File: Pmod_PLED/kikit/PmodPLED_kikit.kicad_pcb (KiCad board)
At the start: 2 copper layers, 86.5 x 99.3 mm, 148 parts, among them IC1 TBD62064APG, IC2 LM2940T-5.0, J1 Barrel_Jack_Switch, J2 Conn_01x06_Pin, J3 Conn_01x03_Pin

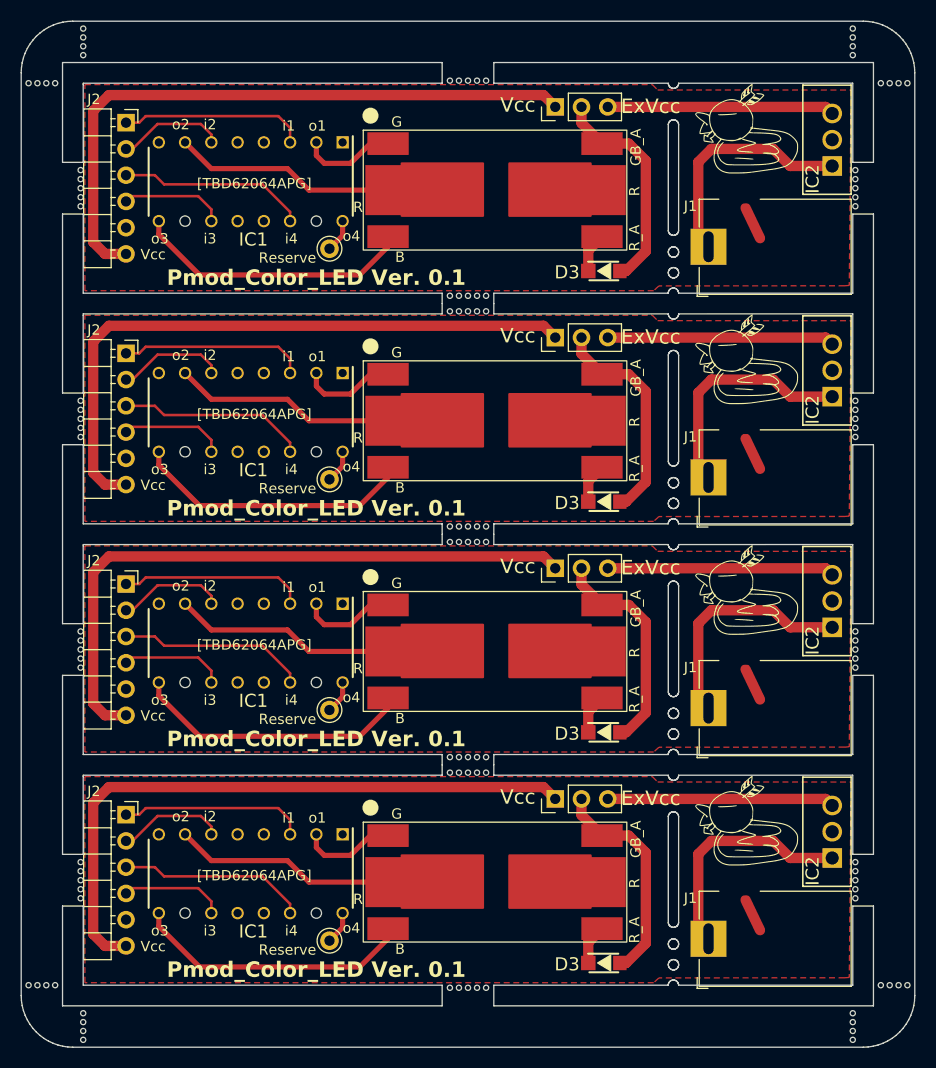
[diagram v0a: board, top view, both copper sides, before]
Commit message: 601d
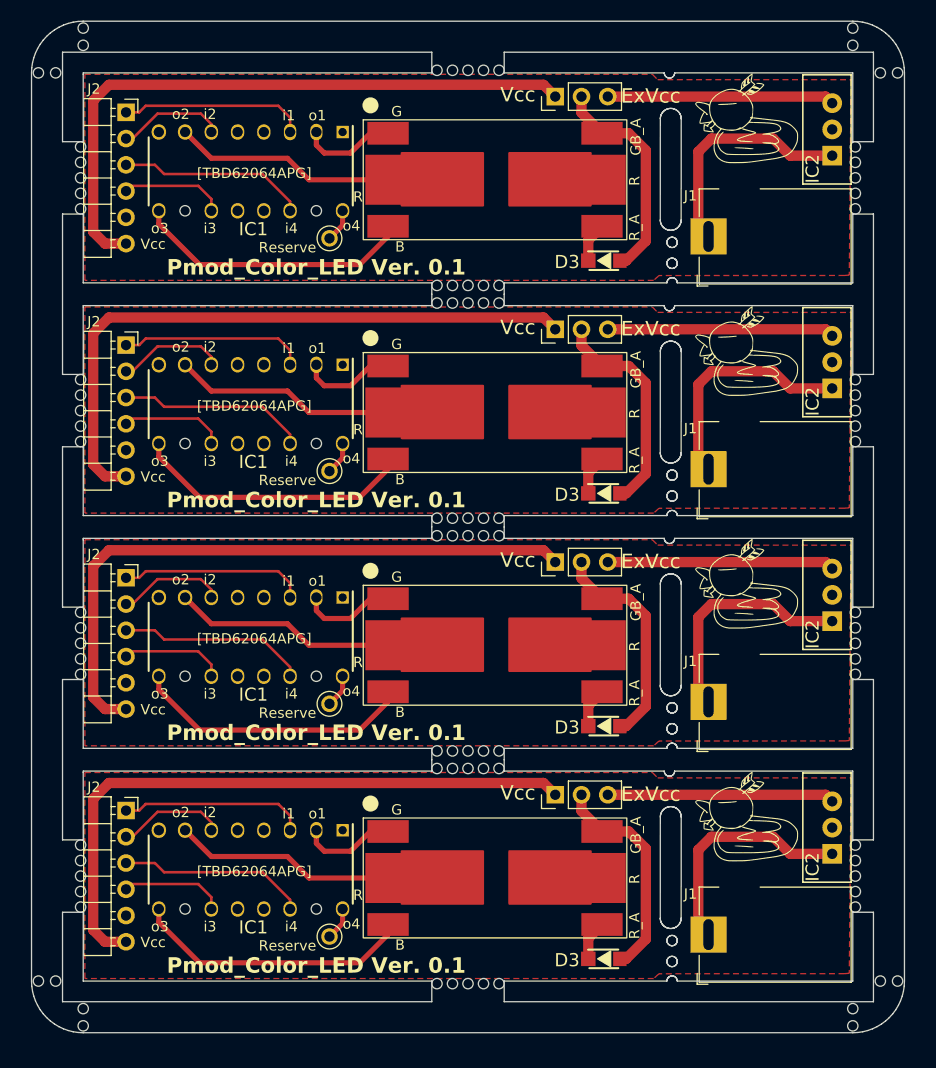
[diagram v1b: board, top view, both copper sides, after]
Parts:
- removed the D1 at (151.2, 36.3)
- removed the D1 at (151.2, 103.3)
- removed the D1 at (151.2, 81.0)
- removed the D1 at (151.2, 58.7)
- removed the D3 at (161.6, 66.5)
- removed the D3 at (161.6, 111.1)
- removed the D3 at (161.6, 88.8)
- removed the D3 at (161.6, 44.2)
- removed the G*** at (175.4, 97.4)
- removed the G*** at (175.4, 75.1)
- removed the G*** at (175.4, 30.5)
- removed the G*** at (175.4, 52.8)
- removed the IC1 at (127.5, 80.2)
- removed the IC1 at (127.5, 35.5)
- removed the IC1 at (127.5, 102.5)
- removed the IC1 at (127.5, 57.9)
- removed the IC2 at (182.7, 95.9)
- removed the IC2 at (182.7, 51.2)
- removed the IC2 at (182.7, 28.9)
- removed the IC2 at (182.7, 73.6)
- removed the J1 at (171.8, 64.1)
- removed the J1 at (171.8, 86.5)
- removed the J1 at (171.8, 108.8)
- removed the J1 at (171.8, 41.8)
- removed the J2 at (111.4, 95.5)
- removed the J2 at (111.4, 73.2)
- removed the J2 at (111.4, 50.9)
- removed the J2 at (111.4, 28.5)
- removed the J3 at (156.9, 28.3)
- removed the J3 at (156.9, 72.9)
- removed the J3 at (156.9, 95.2)
- removed the J3 at (156.9, 50.6)
- removed the REF** at (111.0, 35.3)
- removed the REF** at (186.0, 103.1)
- removed the REF** at (147.6, 70.4)
- removed the REF** at (111.3, 118.6)
- removed the REF** at (150.2, 46.6)
- removed the REF** at (185.7, 118.6)
- removed the REF** at (111.0, 60.2)
- removed the REF** at (111.3, 116.8)
- removed the REF** at (189.3, 113.3)
- removed the REF** at (106.8, 26.0)
- removed the REF** at (149.4, 48.1)
- removed the REF** at (108.6, 113.3)
- removed the REF** at (111.0, 37.0)
- removed the REF** at (186.0, 60.2)
- removed the REF** at (150.2, 92.7)
- removed the REF** at (186.0, 56.7)
- removed the REF** at (150.2, 113.5)
- removed the REF** at (185.7, 23.3)
- removed the REF** at (111.0, 82.5)
- removed the REF** at (108.6, 26.0)
- removed the REF** at (111.0, 102.2)
- removed the REF** at (111.0, 57.6)
- removed the REF** at (147.6, 25.8)
- removed the REF** at (146.8, 70.4)
- removed the REF** at (186.0, 37.9)
- removed the REF** at (189.3, 26.0)
- removed the REF** at (146.8, 25.8)
- removed the REF** at (111.3, 22.4)
- removed the REF** at (107.7, 26.0)
- removed the REF** at (111.3, 23.3)
- removed the REF** at (186.0, 79.0)
- removed the REF** at (111.0, 81.7)
- removed the REF** at (186.0, 59.4)
- removed the REF** at (106.8, 113.3)
- removed the REF** at (185.7, 116.0)
- removed the REF** at (149.4, 70.4)
- removed the REF** at (185.7, 117.7)
- removed the REF** at (148.5, 46.6)
- removed the REF** at (147.6, 48.1)
- removed the REF** at (186.0, 58.5)
- removed the REF** at (111.3, 20.7)
- removed the REF** at (111.0, 79.0)
- removed the REF** at (186.0, 101.4)
- removed the REF** at (111.0, 59.4)
- removed the REF** at (148.5, 113.5)
- removed the REF** at (186.0, 80.8)
- removed the REF** at (186.0, 102.2)
- removed the REF** at (185.7, 20.7)
- removed the REF** at (186.0, 36.2)
- removed the REF** at (146.8, 68.9)
- removed the REF** at (186.0, 104.0)
- removed the REF** at (149.4, 46.6)
- removed the REF** at (147.6, 68.9)
- removed the REF** at (148.5, 91.2)
- removed the REF** at (149.4, 91.2)
- removed the REF** at (185.7, 22.4)
- removed the REF** at (186.0, 37.0)
- removed the REF** at (186.0, 81.7)
- removed the REF** at (106.0, 26.0)
- removed the REF** at (147.6, 91.2)
- removed the REF** at (146.8, 91.2)
- removed the REF** at (186.0, 34.4)
- removed the REF** at (111.3, 117.7)
- removed the REF** at (111.0, 37.9)
- removed the REF** at (191.0, 113.3)
- removed the REF** at (188.4, 26.0)
- removed the REF** at (190.2, 26.0)
- removed the REF** at (146.8, 92.7)
- removed the REF** at (148.5, 25.8)
- removed the REF** at (147.6, 92.7)
- removed the REF** at (185.7, 21.6)
- removed the REF** at (186.0, 82.5)
- removed the REF** at (150.2, 70.4)
- removed the REF** at (111.3, 116.0)
- removed the REF** at (146.8, 48.1)
- removed the REF** at (106.0, 113.3)
- removed the REF** at (107.7, 113.3)
- removed the REF** at (111.3, 21.6)
- removed the REF** at (111.0, 34.4)
- removed the REF** at (190.2, 113.3)
- removed the REF** at (147.6, 113.5)
- removed the REF** at (185.7, 116.8)
- removed the REF** at (148.5, 48.1)
- removed the REF** at (191.0, 26.0)
- removed the REF** at (111.0, 36.2)
- removed the REF** at (186.0, 79.9)
- removed the REF** at (186.0, 57.6)
- removed the REF** at (111.0, 80.8)
- removed the REF** at (186.0, 35.3)
- removed the REF** at (147.6, 46.6)
- removed the REF** at (146.8, 46.6)
- removed the REF** at (146.8, 113.5)
- removed the REF** at (111.0, 56.7)
- removed the REF** at (111.0, 58.5)
- removed the REF** at (111.0, 104.9)
- removed the REF** at (150.2, 68.9)
- removed the REF** at (150.2, 48.1)
- removed the REF** at (148.5, 70.4)
- removed the REF** at (149.4, 92.7)
- removed the REF** at (111.0, 103.1)
- removed the REF** at (111.0, 101.4)
- removed the REF** at (149.4, 68.9)
- removed the REF** at (111.0, 104.0)
- removed the REF** at (188.4, 113.3)
- removed the REF** at (186.0, 104.9)
- removed the REF** at (111.0, 79.9)
- removed the REF** at (149.4, 25.8)
- removed the REF** at (150.2, 25.8)
- removed the REF** at (148.5, 68.9)
- removed the REF** at (148.5, 92.7)
- removed the REF** at (149.4, 113.5)
- removed the REF** at (150.2, 91.2)
- removed the Reserve at (135.1, 109.0)
- removed the Reserve at (135.1, 64.3)
- removed the Reserve at (135.1, 86.6)
- removed the Reserve at (135.1, 42.0)
- added D1: EP204K-150G1R1B1-CA, MyLibrary:EP204-150G1R1B1-CA, F.Cu at (151.2, 102.9)
- added D1: EP204K-150G1R1B1-CA, MyLibrary:EP204-150G1R1B1-CA, F.Cu at (151.2, 35.3)
- added D1: EP204K-150G1R1B1-CA, MyLibrary:EP204-150G1R1B1-CA, F.Cu at (151.2, 57.9)
- added D1: EP204K-150G1R1B1-CA, MyLibrary:EP204-150G1R1B1-CA, F.Cu at (151.2, 80.4)
- added D3: SS2040FL, SamacSys_Parts:SODFL3618X108N, F.Cu at (161.6, 110.7)
- added D3: SS2040FL, SamacSys_Parts:SODFL3618X108N, F.Cu at (161.6, 43.2)
- added D3: SS2040FL, SamacSys_Parts:SODFL3618X108N, F.Cu at (161.6, 88.2)
- added D3: SS2040FL, SamacSys_Parts:SODFL3618X108N, F.Cu at (161.6, 65.7)
- added G***: LOGO, MyLibrary:logo_kamo_ss, F.Cu at (175.4, 74.5)
- added G***: LOGO, MyLibrary:logo_kamo_ss, F.Cu at (175.4, 97.0)
- added G***: LOGO, MyLibrary:logo_kamo_ss, F.Cu at (175.4, 52.0)
- added G***: LOGO, MyLibrary:logo_kamo_ss, F.Cu at (175.4, 29.5)
- added IC1: TBD62064APG, SamacSys_Parts:DIP762W60P254L1975H445Q16N, F.Cu at (127.5, 34.5)
- added IC1: TBD62064APG, SamacSys_Parts:DIP762W60P254L1975H445Q16N, F.Cu at (127.5, 79.6)
- added IC1: TBD62064APG, SamacSys_Parts:DIP762W60P254L1975H445Q16N, F.Cu at (127.5, 57.1)
- added IC1: TBD62064APG, SamacSys_Parts:DIP762W60P254L1975H445Q16N, F.Cu at (127.5, 102.1)
- added IC2: LM2940T-5.0, SamacSys_Parts:TO254P470X1016X2222-3P, F.Cu at (182.7, 95.5)
- added IC2: LM2940T-5.0, SamacSys_Parts:TO254P470X1016X2222-3P, F.Cu at (182.7, 50.4)
- added IC2: LM2940T-5.0, SamacSys_Parts:TO254P470X1016X2222-3P, F.Cu at (182.7, 27.9)
- added IC2: LM2940T-5.0, SamacSys_Parts:TO254P470X1016X2222-3P, F.Cu at (182.7, 73.0)
- added J1: Barrel_Jack_Switch, Connector_BarrelJack:BarrelJack_Horizontal, F.Cu at (171.8, 63.3)
- added J1: Barrel_Jack_Switch, Connector_BarrelJack:BarrelJack_Horizontal, F.Cu at (171.8, 108.4)
- added J1: Barrel_Jack_Switch, Connector_BarrelJack:BarrelJack_Horizontal, F.Cu at (171.8, 85.9)
- added J1: Barrel_Jack_Switch, Connector_BarrelJack:BarrelJack_Horizontal, F.Cu at (171.8, 40.8)
- added J2: Conn_01x06_Pin, Library:Pmod6, F.Cu at (111.4, 72.6)
- added J2: Conn_01x06_Pin, Library:Pmod6, F.Cu at (111.4, 50.1)
- added J2: Conn_01x06_Pin, Library:Pmod6, F.Cu at (111.4, 95.1)
- added J2: Conn_01x06_Pin, Library:Pmod6, F.Cu at (111.4, 27.5)
- added J3: Conn_01x03_Pin, Connector_PinHeader_2.54mm:PinHeader_1x03_P2.54mm_Vertical, F.Cu at (156.9, 94.8)
- added J3: Conn_01x03_Pin, Connector_PinHeader_2.54mm:PinHeader_1x03_P2.54mm_Vertical, F.Cu at (156.9, 49.8)
- added J3: Conn_01x03_Pin, Connector_PinHeader_2.54mm:PinHeader_1x03_P2.54mm_Vertical, F.Cu at (156.9, 27.3)
- added J3: Conn_01x03_Pin, Connector_PinHeader_2.54mm:PinHeader_1x03_P2.54mm_Vertical, F.Cu at (156.9, 72.3)
- added REF**: NPTH, NPTH, F.Cu at (186.0, 59.2)
- added REF**: NPTH, NPTH, F.Cu at (186.0, 60.7)
- added REF**: NPTH, NPTH, F.Cu at (186.0, 33.7)
- added REF**: NPTH, NPTH, F.Cu at (111.0, 35.2)
- added REF**: NPTH, NPTH, F.Cu at (150.0, 24.8)
- added REF**: NPTH, NPTH, F.Cu at (185.7, 115.5)
- added REF**: NPTH, NPTH, F.Cu at (150.0, 68.1)
- added REF**: NPTH, NPTH, F.Cu at (190.1, 25.0)
- added REF**: NPTH, NPTH, F.Cu at (111.3, 20.7)
- added REF**: NPTH, NPTH, F.Cu at (111.0, 99.7)
- added REF**: NPTH, NPTH, F.Cu at (111.0, 56.2)
- added REF**: NPTH, NPTH, F.Cu at (145.5, 90.6)
- added REF**: NPTH, NPTH, F.Cu at (111.0, 57.7)
- added REF**: NPTH, NPTH, F.Cu at (106.9, 25.0)
- added REF**: NPTH, NPTH, F.Cu at (111.0, 105.7)
- added REF**: NPTH, NPTH, F.Cu at (151.5, 24.8)
- added REF**: NPTH, NPTH, F.Cu at (111.0, 78.7)
- added REF**: NPTH, NPTH, F.Cu at (111.3, 117.2)
- added REF**: NPTH, NPTH, F.Cu at (150.0, 45.6)
- added REF**: NPTH, NPTH, F.Cu at (147.0, 69.8)
- added REF**: NPTH, NPTH, F.Cu at (185.7, 22.3)
- added REF**: NPTH, NPTH, F.Cu at (151.5, 47.3)
- added REF**: NPTH, NPTH, F.Cu at (186.0, 36.7)
- added REF**: NPTH, NPTH, F.Cu at (186.0, 56.2)
- added REF**: NPTH, NPTH, F.Cu at (148.5, 92.3)
- added REF**: NPTH, NPTH, F.Cu at (148.5, 45.6)
- added REF**: NPTH, NPTH, F.Cu at (147.0, 92.3)
- added REF**: NPTH, NPTH, F.Cu at (147.0, 24.8)
- added REF**: NPTH, NPTH, F.Cu at (145.5, 45.6)
- added REF**: NPTH, NPTH, F.Cu at (147.0, 45.6)
- added REF**: NPTH, NPTH, F.Cu at (150.0, 92.3)
- added REF**: NPTH, NPTH, F.Cu at (188.4, 112.9)
- added REF**: NPTH, NPTH, F.Cu at (106.9, 112.9)
- added REF**: NPTH, NPTH, F.Cu at (145.5, 92.3)
- added REF**: NPTH, NPTH, F.Cu at (186.0, 99.7)
- added REF**: NPTH, NPTH, F.Cu at (145.5, 113.1)
- added REF**: NPTH, NPTH, F.Cu at (111.3, 22.3)
- added REF**: NPTH, NPTH, F.Cu at (111.0, 81.7)
- added REF**: NPTH, NPTH, F.Cu at (186.0, 101.2)
- added REF**: NPTH, NPTH, F.Cu at (111.3, 115.5)
- added REF**: NPTH, NPTH, F.Cu at (151.5, 69.8)
- added REF**: NPTH, NPTH, F.Cu at (188.4, 25.0)
- added REF**: NPTH, NPTH, F.Cu at (111.0, 59.2)
- added REF**: NPTH, NPTH, F.Cu at (186.0, 105.7)
- added REF**: NPTH, NPTH, F.Cu at (148.5, 69.8)
- added REF**: NPTH, NPTH, F.Cu at (147.0, 90.6)
- added REF**: NPTH, NPTH, F.Cu at (147.0, 47.3)
- added REF**: NPTH, NPTH, F.Cu at (186.0, 78.7)
- added REF**: NPTH, NPTH, F.Cu at (150.0, 47.3)
- added REF**: NPTH, NPTH, F.Cu at (111.0, 54.7)
- added REF**: NPTH, NPTH, F.Cu at (186.0, 35.2)
- added REF**: NPTH, NPTH, F.Cu at (145.5, 69.8)
- added REF**: NPTH, NPTH, F.Cu at (111.0, 83.2)
- added REF**: NPTH, NPTH, F.Cu at (111.0, 104.2)
- added REF**: NPTH, NPTH, F.Cu at (151.5, 90.6)
- added REF**: NPTH, NPTH, F.Cu at (111.0, 80.2)
- added REF**: NPTH, NPTH, F.Cu at (111.0, 102.7)
- added REF**: NPTH, NPTH, F.Cu at (111.0, 60.7)
- added REF**: NPTH, NPTH, F.Cu at (186.0, 38.2)
- added REF**: NPTH, NPTH, F.Cu at (145.5, 24.8)
- added REF**: NPTH, NPTH, F.Cu at (111.0, 32.2)
- added REF**: NPTH, NPTH, F.Cu at (148.5, 90.6)
- added REF**: NPTH, NPTH, F.Cu at (186.0, 102.7)
- added REF**: NPTH, NPTH, F.Cu at (108.6, 112.9)
- added REF**: NPTH, NPTH, F.Cu at (186.0, 80.2)
- added REF**: NPTH, NPTH, F.Cu at (151.5, 92.3)
- added REF**: NPTH, NPTH, F.Cu at (150.0, 90.6)
- added REF**: NPTH, NPTH, F.Cu at (145.5, 68.1)
- added REF**: NPTH, NPTH, F.Cu at (186.0, 81.7)
- added REF**: NPTH, NPTH, F.Cu at (186.0, 32.2)
- added REF**: NPTH, NPTH, F.Cu at (148.5, 113.1)
- added REF**: NPTH, NPTH, F.Cu at (190.1, 112.9)
- added REF**: NPTH, NPTH, F.Cu at (145.5, 47.3)
- added REF**: NPTH, NPTH, F.Cu at (151.5, 113.1)
- added REF**: NPTH, NPTH, F.Cu at (185.7, 117.2)
- added REF**: NPTH, NPTH, F.Cu at (111.0, 38.2)
- added REF**: NPTH, NPTH, F.Cu at (111.0, 36.7)
- added REF**: NPTH, NPTH, F.Cu at (147.0, 68.1)
- added REF**: NPTH, NPTH, F.Cu at (108.6, 25.0)
- added REF**: NPTH, NPTH, F.Cu at (151.5, 68.1)
- added REF**: NPTH, NPTH, F.Cu at (186.0, 83.2)
- added REF**: NPTH, NPTH, F.Cu at (186.0, 104.2)
- added REF**: NPTH, NPTH, F.Cu at (151.5, 45.6)
- added REF**: NPTH, NPTH, F.Cu at (148.5, 68.1)
- added REF**: NPTH, NPTH, F.Cu at (111.0, 33.7)
- added REF**: NPTH, NPTH, F.Cu at (148.5, 47.3)
- added REF**: NPTH, NPTH, F.Cu at (150.0, 69.8)
- added REF**: NPTH, NPTH, F.Cu at (150.0, 113.1)
- added REF**: NPTH, NPTH, F.Cu at (111.0, 101.2)
- added REF**: NPTH, NPTH, F.Cu at (186.0, 57.7)
- added REF**: NPTH, NPTH, F.Cu at (147.0, 113.1)
- added REF**: NPTH, NPTH, F.Cu at (186.0, 54.7)
- added REF**: NPTH, NPTH, F.Cu at (111.0, 77.2)
- added REF**: NPTH, NPTH, F.Cu at (185.7, 20.7)
- added REF**: NPTH, NPTH, F.Cu at (148.5, 24.8)
- added REF**: NPTH, NPTH, F.Cu at (186.0, 77.2)
- added Reserve: TestPoint, TestPoint:TestPoint_Pad_D2.0mm, F.Cu at (135.1, 108.6)
- added Reserve: TestPoint, TestPoint:TestPoint_Pad_D2.0mm, F.Cu at (135.1, 41.0)
- added Reserve: TestPoint, TestPoint:TestPoint_Pad_D2.0mm, F.Cu at (135.1, 86.0)
- added Reserve: TestPoint, TestPoint:TestPoint_Pad_D2.0mm, F.Cu at (135.1, 63.5)
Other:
- board size 86.5 x 99.3 mm -> 84.5 x 97.9 mm
